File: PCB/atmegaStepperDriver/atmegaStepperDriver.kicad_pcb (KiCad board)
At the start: 2 copper layers, 51.4 x 92.1 mm, 74 parts, among them J1 General power, J2 Motor Output, J3 Motor power, J4 Conn_01x05_Socket, J5 Reset Header, J6 I2C Communication pins, J9 Stepper communication pins, Q1 TIP42C, Q10 BC547, Q11 BC557, Q12 BC547, Q13 BC557, Q14 BC547, Q15 BC557, Q16 BC547, Q2 TIP41C, Q3 TIP42C, Q4 TIP42C, Q5 TIP42C, Q6 TIP41C, Q7 TIP41C, Q8 TIP41C, Q9 BC557, U1 ATmega328P-P, U2 LM7805_TO220, Y1 Crystal

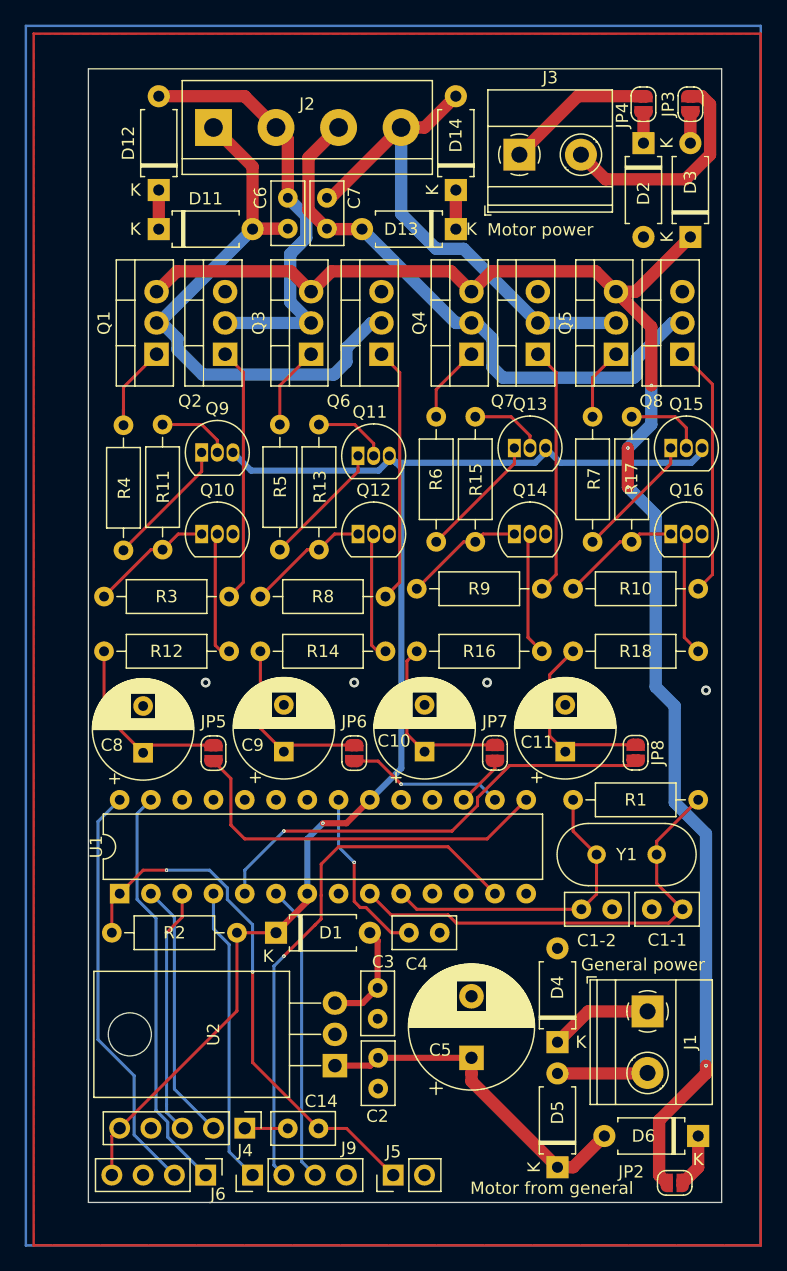
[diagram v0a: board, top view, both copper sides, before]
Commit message: fixed old design flaw; full redisgn; Few things to be done; V0.8.0;
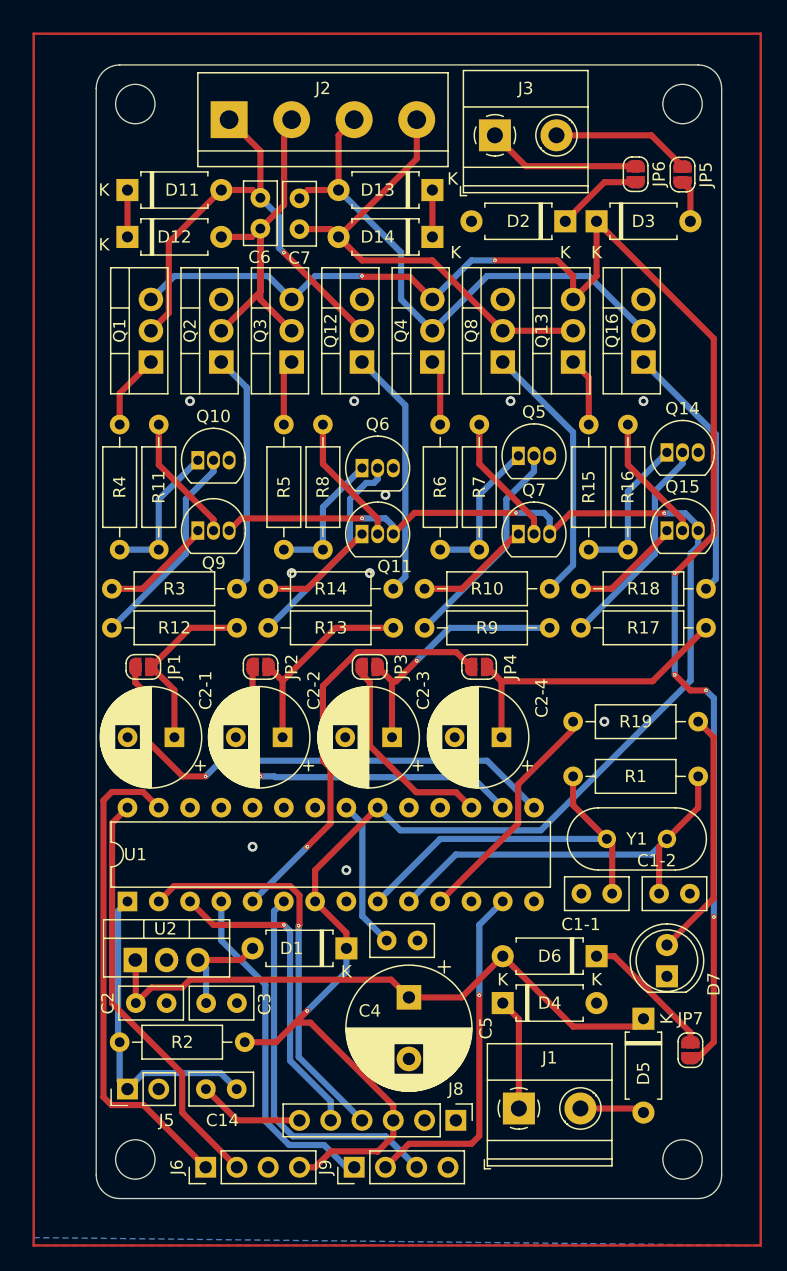
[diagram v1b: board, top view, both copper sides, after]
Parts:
- removed C10, C11, C8, C9: C, Capacitor_THT:CP_Radial_D8.0mm_P3.80mm
- removed J4: Conn_01x05_Socket, Connector_PinHeader_2.54mm:PinHeader_1x05_P2.54mm_Vertical
- removed JP8: SolderJumper_2_Open, Jumper:SolderJumper-2_P1.3mm_Open_RoundedPad1.0x1.5mm
- added C2-1: C, Capacitor_THT:CP_Radial_D8.0mm_P3.80mm, F.Cu at (72.4, 99.7)
- added C2-2: C, Capacitor_THT:CP_Radial_D8.0mm_P3.80mm, F.Cu at (81.2, 99.7)
- added C2-3: C, Capacitor_THT:CP_Radial_D8.0mm_P3.80mm, F.Cu at (90.1, 99.7)
- added C2-4: C, Capacitor_THT:CP_Radial_D8.0mm_P3.80mm, F.Cu at (99.0, 99.7)
- added D7: LED, LED_THT:LED_D5.0mm, F.Cu at (112.4, 119.1)
- added J8: Conn_01x06_Socket, Connector_PinHeader_2.54mm:PinHeader_1x06_P2.54mm_Vertical, F.Cu at (95.2, 130.8)
- added JP1: SolderJumper_2_Open, Jumper:SolderJumper-2_P1.3mm_Open_RoundedPad1.0x1.5mm, F.Cu at (69.9, 94.0)
- added R19: 220, Resistor_THT:R_Axial_DIN0207_L6.3mm_D2.5mm_P10.16mm_Horizontal, F.Cu at (104.8, 98.4)
- added REF**: MountingHole_3.2mm_M3_DIN965, MountingHole:MountingHole_3.2mm_M3_DIN965, F.Cu at (113.7, 48.3)
- added REF**: MountingHole_3.2mm_M3_DIN965, MountingHole:MountingHole_3.2mm_M3_DIN965, F.Cu at (113.7, 134.0)
- added REF**: MountingHole_3.2mm_M3_DIN965, MountingHole:MountingHole_3.2mm_M3_DIN965, F.Cu at (69.2, 134.0)
- added REF**: MountingHole_3.2mm_M3_DIN965, MountingHole:MountingHole_3.2mm_M3_DIN965, F.Cu at (69.2, 48.3)
- Q12, Q16: value BC547 -> TIP41C; footprint Package_TO_SOT_THT:TO-92_Inline -> Package_TO_SOT_THT:TO-220-3_Vertical
- Q13: value BC557 -> TIP42C; footprint Package_TO_SOT_THT:TO-92_Inline -> Package_TO_SOT_THT:TO-220-3_Vertical
- Q5: value TIP42C -> BC547; footprint Package_TO_SOT_THT:TO-220-3_Vertical -> Package_TO_SOT_THT:TO-92_Inline
- Q6: value TIP41C -> BC547; footprint Package_TO_SOT_THT:TO-220-3_Vertical -> Package_TO_SOT_THT:TO-92_Inline
- Q7: value TIP41C -> BC557; footprint Package_TO_SOT_THT:TO-220-3_Vertical -> Package_TO_SOT_THT:TO-92_Inline
- R14, R15, R18: value 1k -> 50
- R7, R8, R9: value 50 -> 1k
- U2: footprint Package_TO_SOT_THT:TO-220-3_Horizontal_TabDown -> Package_TO_SOT_THT:TO-220-3_Vertical
- moved JP5 60.5 mm to (113.7, 54.0), turned to 90 degrees
- moved JP2 53.7 mm to (79.4, 94.0), turned to 180 degrees
- moved JP3 52.6 mm to (88.2, 94.0), turned to 180 degrees
- moved JP6 52.3 mm to (109.9, 54.0), turned to 90 degrees
- moved JP4 47.6 mm to (97.1, 94.0), turned to 180 degrees
- moved JP7 28.9 mm to (114.3, 125.1), turned to 90 degrees
- moved J5 22.7 mm to (68.6, 128.3)
- moved R16 19.0 mm to (109.2, 84.5), turned to 90 degrees
- moved C2 18.5 mm to (71.8, 121.3), turned to 180 degrees
- moved U2 18.3 mm to (69.2, 117.8), turned to 0 degrees
- moved D6 16.8 mm to (106.7, 117.5)
- moved Q7 14.7 mm to (100.3, 83.2), turned to 0 degrees
- moved Q8 14.6 mm to (99.1, 69.2)
- moved Q16 14.1 mm to (110.5, 69.2), turned to 90 degrees
- moved Q14 14.1 mm to (112.4, 76.6)
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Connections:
- JP2 pad 1: Motor Power -> Gate 2
- JP2 pad 2: Net-(D6-K) -> Net-(JP2-B)
- JP3 pad 1: Net-(D3-A) -> Gate 3
- JP3 pad 2: Net-(J3-Pin_2) -> Net-(JP3-B)
- JP4 pad 1: Net-(D2-K) -> Gate 4
- JP4 pad 2: Net-(J3-Pin_1) -> Jumper To lower Pins
- JP5 pad 1: Gate 1 -> Net-(D3-A)
- JP5 pad 2: Net-(JP5-B) -> Net-(J3-Pin_2)
- JP6 pad 1: Gate 2 -> Net-(D2-K)
- JP6 pad 2: Net-(JP6-B) -> Net-(J3-Pin_1)
- JP7 pad 1: Gate 3 -> Motor Power
- JP7 pad 2: Net-(JP7-B) -> Net-(D6-K)
- Q12 pad 1: Net-(Q12-C) -> Net-(Q12-B)
- Q12 pad 2: Net-(Q12-B) -> output A
- Q13 pad 1: Net-(Q13-C) -> Net-(Q13-B)
- Q13 pad 2: Net-(Q13-B) -> output !B
- Q13 pad 3: +5V -> Motor Power
- Q16 pad 1: Net-(Q16-C) -> Net-(Q16-B)
- Q16 pad 2: Net-(Q16-B) -> output B
- Q5 pad 1: Net-(Q5-B) -> Net-(Q5-C)
- Q5 pad 2: output !B -> Net-(Q5-B)
- Q5 pad 3: Motor Power -> GND
- Q6 pad 1: Net-(Q6-B) -> Net-(Q6-C)
- Q6 pad 2: output A -> Net-(Q6-B)
- Q7 pad 1: Net-(Q7-B) -> Net-(Q7-C)
- Q7 pad 2: output !B -> Net-(Q7-B)
- Q7 pad 3: GND -> +5V
- Q8 pad 2: output B -> output !B
- R10 pad 1: Net-(Q16-C) -> Net-(Q7-C)
- R13 pad 1: Net-(Q12-C) -> Gate 2
- R13 pad 2: Net-(Q11-B) -> Net-(Q6-B)
- R14 pad 1: Gate 2 -> Net-(Q11-C)
- R15 pad 1: Net-(Q14-C) -> Net-(Q13-B)
- R15 pad 2: Net-(Q13-B) -> Net-(Q14-C)
- R16 pad 1: Gate 3 -> Net-(Q14-C)
- R16 pad 2: Net-(Q14-B) -> Net-(Q15-B)
- R17 pad 1: Net-(Q16-C) -> Gate 4
- R17 pad 2: Net-(Q15-B) -> Net-(Q14-B)
- R18 pad 1: Gate 4 -> Net-(Q15-C)
- R3 pad 1: Net-(Q10-C) -> Net-(Q9-C)
- R4 pad 2: Net-(Q9-C) -> Net-(Q10-C)
- R5 pad 1: Net-(Q11-C) -> Net-(Q3-B)
- R5 pad 2: Net-(Q3-B) -> Net-(Q6-C)
- R6 pad 2: Net-(Q13-C) -> Net-(Q5-C)
- R7 pad 1: Net-(Q15-C) -> Net-(Q5-C)
- R7 pad 2: Net-(Q5-B) -> Net-(Q7-B)
- R8 pad 1: Net-(Q12-C) -> Net-(Q6-C)
- R8 pad 2: Net-(Q6-B) -> Net-(Q11-B)
- R9 pad 1: Net-(Q14-C) -> Gate 3
- R9 pad 2: Net-(Q7-B) -> Net-(Q5-B)
- U1 pad 11: unconnected-(U1-PD5-Pad11) -> Net-(U1-PD5)
- U1 pad 15: Net-(JP5-B) -> Net-(JP1-B)
- U1 pad 16: Net-(JP6-B) -> Net-(JP2-B)
- U1 pad 17: Net-(JP7-B) -> Net-(JP3-B)
- U1 pad 2: TX -> RXD
- U1 pad 3: RX -> TXD
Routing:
- net Net-(JP1-B): track 0.00 -> 41.1 mm, vias 0 -> 1
- net RXD: track 0.00 -> 32.7 mm, vias 0 -> 1
- net Net-(JP5-B): track 31.5 -> 0.00 mm
- net Net-(JP2-B): track 0.00 -> 29.9 mm, vias 0 -> 1
- net TXD: track 0.00 -> 25.9 mm, vias 0 -> 1
- net +5V: track 113.1 -> 135.7 mm, vias 1 -> 4
- net VCCInput: track 28.0 -> 50.2 mm
- net TX: track 21.2 -> 0.00 mm
- net Net-(D7-A): track 0.00 -> 20.2 mm
- net RX: track 20.1 -> 0.00 mm, vias 1 -> 0
- net Net-(U1-PD5): track 0.00 -> 19.1 mm
- net RST: track 43.8 -> 25.8 mm, vias 2 -> 0
- net Net-(JP3-B): track 0.00 -> 17.0 mm
- net Rotation: track 43.5 -> 28.5 mm
- net Net-(JP6-B): track 12.7 -> 0.00 mm, vias 1 -> 0
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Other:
- board size 51.4 x 92.1 mm -> 50.8 x 92.1 mm
- board text added: "General Power"
- board text removed: "General power"
- board text removed: "Motor from general"
- board text removed: "atMega Stepper Driver Developer board V0.7.1"
